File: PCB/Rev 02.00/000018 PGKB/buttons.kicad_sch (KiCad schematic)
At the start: 22 parts, among them U12 SN74HCS365PWR

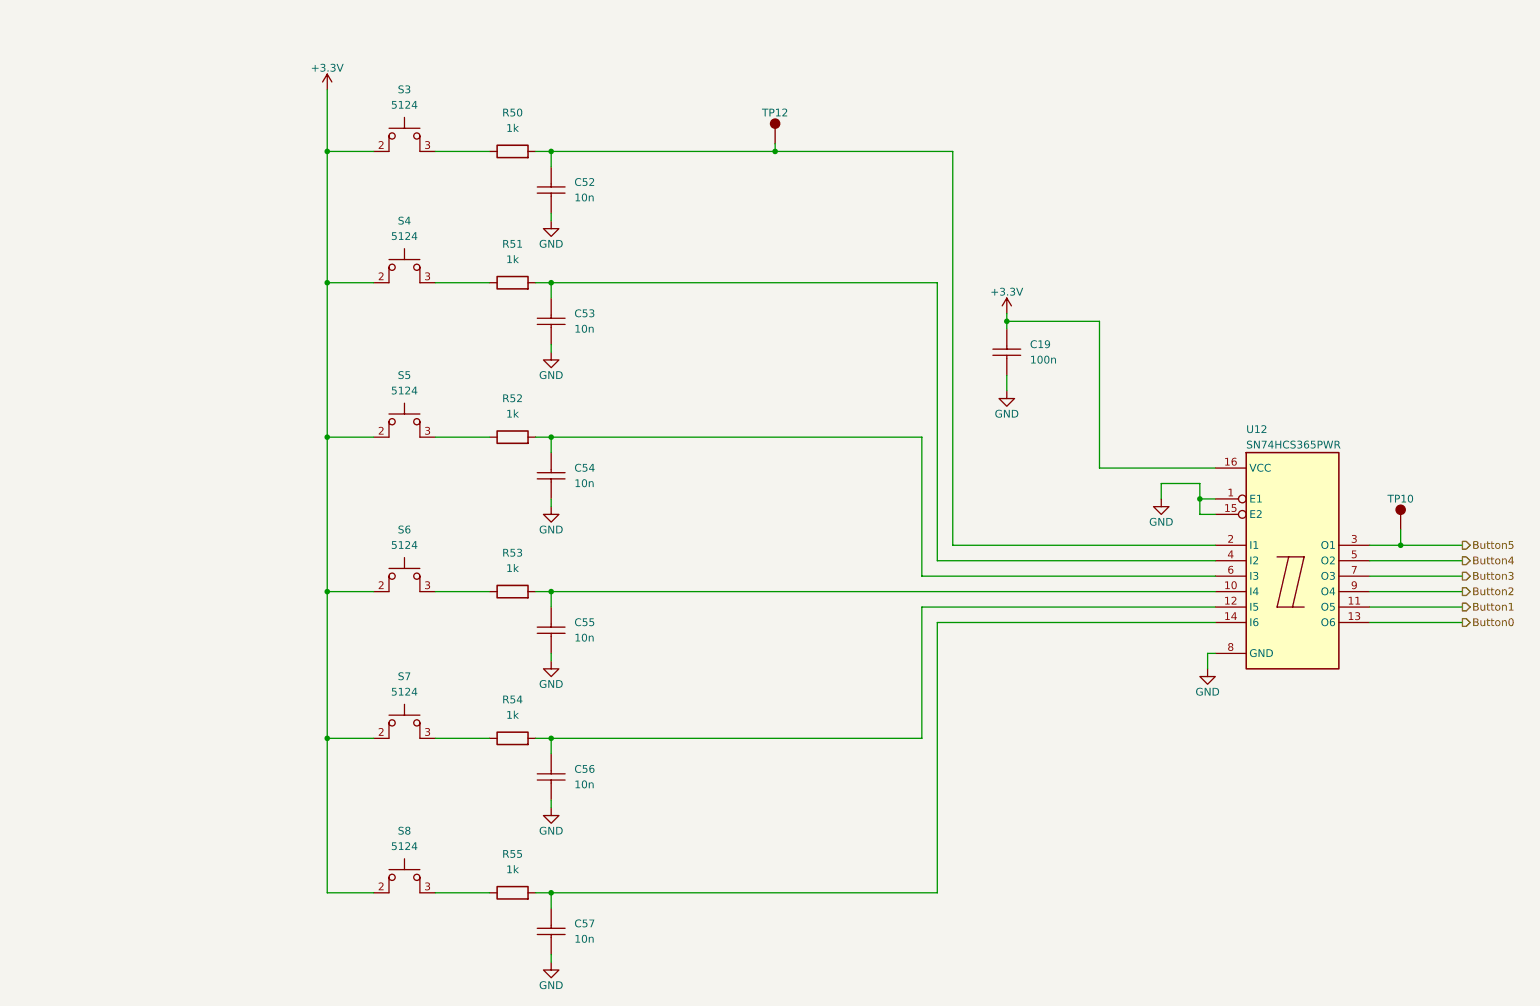
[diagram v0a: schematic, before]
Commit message: ledit
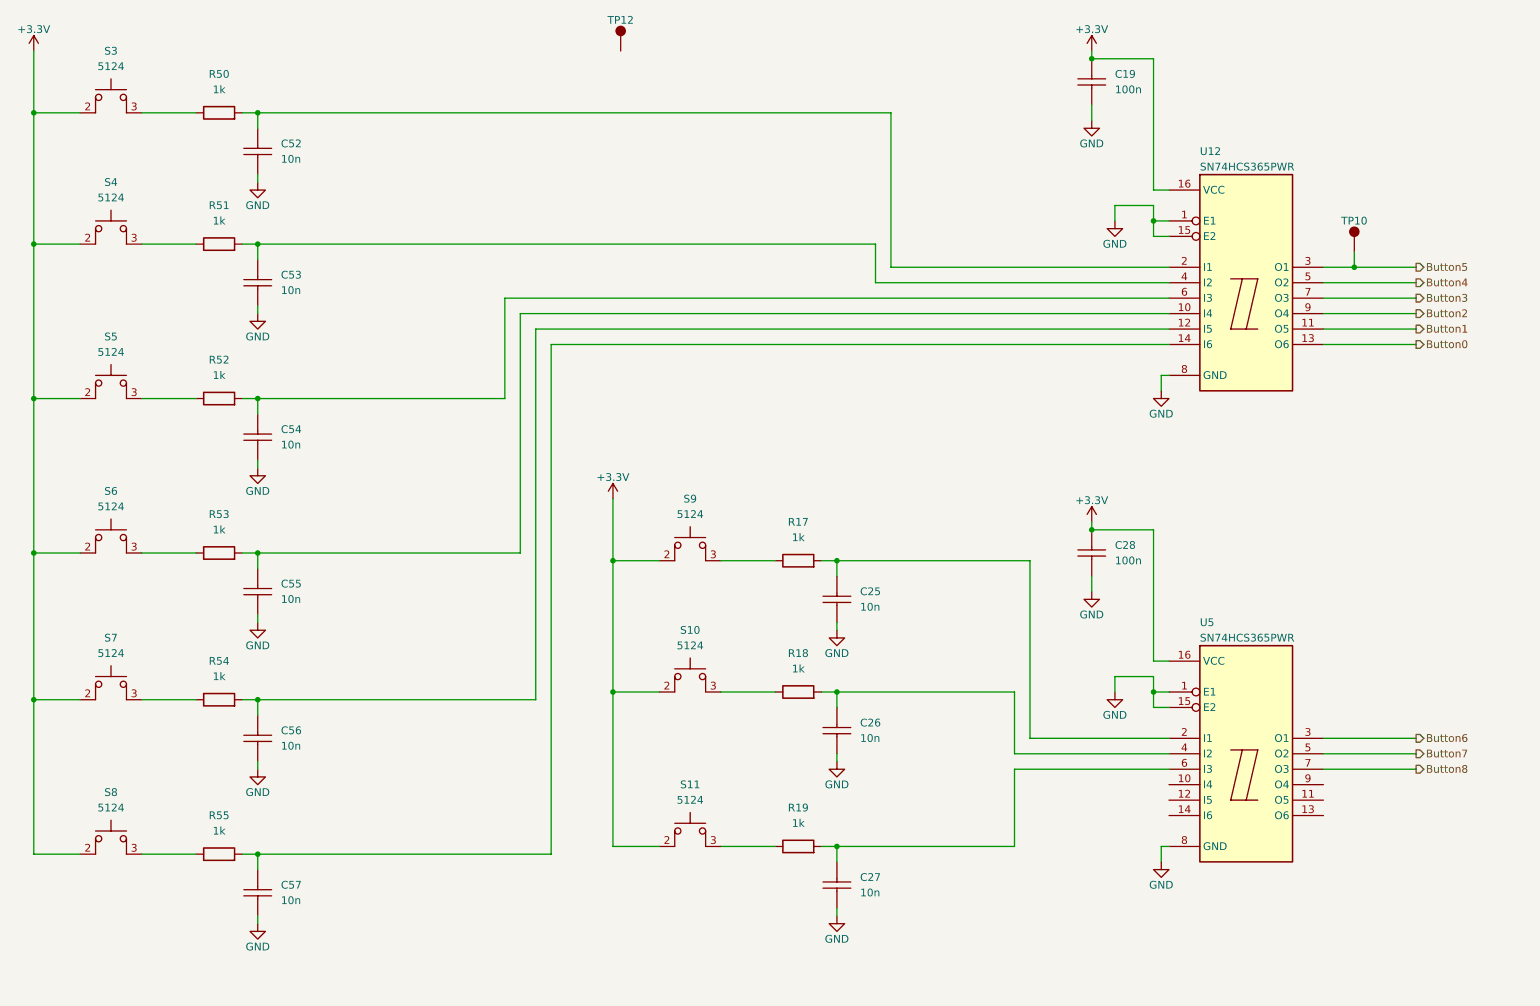
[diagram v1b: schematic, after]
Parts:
- added C25, C26, C27: 10n, KD_Capacitor:CAPC1608X90N, symbol KD_Capacitor:C_0603_10n_X7R_100V
- added C28: 100n, KD_Capacitor:CAPC1608X90N, symbol KD_Capacitor:C_0603_100n_X7R_50V
- added R17, R18, R19: 1k, KD_Resistor:RESC1608X55N, symbol KD_Resistor:R_0603_1k_1%
- added S10, S11, S9: 5124, KD_Switch:SWITCH_BUTTON_Kailh_mx, symbol KD_Switch:Button_keyboard_Adafruit_5124
- added U5: SN74HCS365PWR, KD_Package_SO:SOP65P600X150-16N, symbol KD_IC_Buffer_Driver_Interface:Schmitt_6CH_SN74HCS365PWR
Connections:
- net +3.3V: now also C28.1, S10.2, S11.2, S9.2, U5.16 (VCC)
- net GND: now also C25.2, C26.2, C27.2, C28.2, U5.1 (E1), U5.15 (E2), U5.8 (GND)
- net at C52.1, R50.2, U12.2 (I1): no longer TP12.1
- new net: R17.1, S9.3
- new net: C25.1, R17.2, U5.2 (I1)
- new net: C26.1, R18.2, U5.4 (I2)
- new net: C27.1, R19.2, U5.6 (I3)
- new net: R18.1, S10.3
- new net: R19.1, S11.3
- new net Button6: U5.3 (O1)
- new net Button7: U5.5 (O2)
- new net Button8: U5.7 (O3)
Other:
- moved on the sheet: C19, C52, C53, C54, C55, C56, C57, R50, R51, R52, R53, R54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
